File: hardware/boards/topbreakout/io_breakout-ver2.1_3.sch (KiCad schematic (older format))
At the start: 5 parts, among them J1 WURTH_ELECTRONICS_61400413321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, J2 MOLEX_52892-3033MOLEX_52892-3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, J3 USB-A-S-X-X-VT

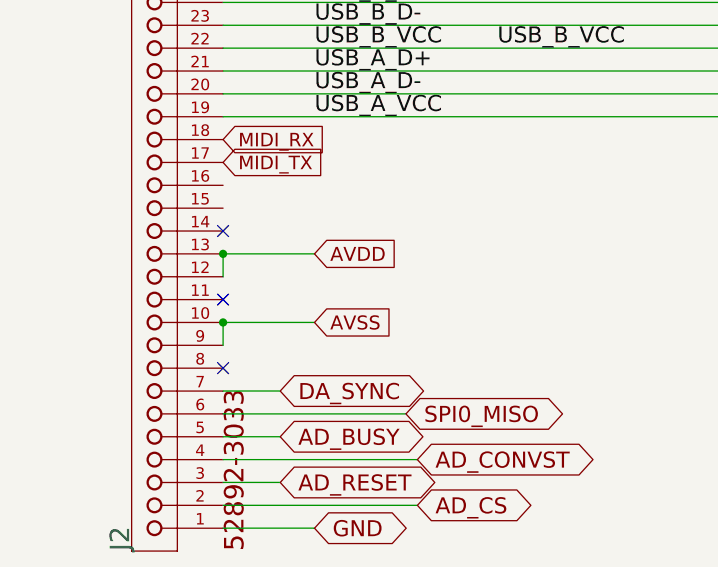
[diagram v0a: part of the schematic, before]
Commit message: refactor
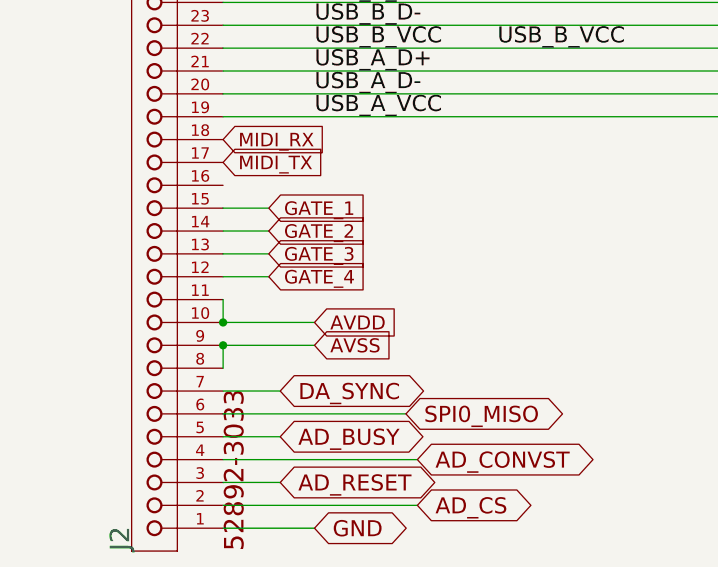
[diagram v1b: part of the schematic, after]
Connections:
- net AVDD: now also J2.10, J2.11; no longer J2.12, J2.13
- net AVSS: now also J2.8; no longer J2.10
- net GATE_2: now reaches J2.14
- net GATE_1: now reaches J2.15
- new net GATE_3: J2.13
- new net GATE_4: J2.12
- no-connect marks 3 -> 0
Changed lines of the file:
@@
-$EndComp
-$Comp
-L TopBreakout-eagle-import:MOLEX_52892-3033MOLEX_52892-3033_0_0 J2
-U 1 1 F1780596
-P 800 6100
-AR Path="/F1780596" Ref="J2"  Part="1"
-AR Path="/5D7F42FA/F1780596" Ref="J2"  Part="1"
-F 0 "J2" H 800 6000 85  0000 L TNN
-F 1 "MOLEX_52892-3033MOLEX_52892-3033_0_0" H 800 6100 50  0001 C CNN
-F 2 "topbreakout:MOLEX_52892-3033_0" H 800 6100 50  0001 C CNN
-F 3 "" H 800 6100 50  0001 C CNN
-	1    800  6100
-	0    -1   -1   0
 $EndComp
 $Comp
@@
 Wire Wire Line
 	5000 5800 6100 5800
-Wire Wire Line
-	1400 5200 1400 5100
-Wire Wire Line
-	1400 4900 1400 4800
-Wire Wire Line
-	1400 4800 1800 4800
-Connection ~ 1400 4800
-Wire Wire Line
-	1400 5100 1800 5100
-Connection ~ 1400 5100
-NoConn ~ 1400 5300
-NoConn ~ 1400 5000
-NoConn ~ 1400 4700
-Text GLabel 1800 4800 2    61   Input ~ 0
+Text GLabel 1800 5100 2    61   Input ~ 0
 AVDD
-Text GLabel 1800 5100 2    61   Input ~ 0
+Text GLabel 1800 5200 2    61   Input ~ 0
 AVSS
 Text GLabel 1400 4300 2    59   Input ~ 0
@@
 Text GLabel 1400 4400 2    59   Input ~ 0
 MIDI_TX
+$Comp
+L TopBreakout-eagle-import:MOLEX_52892-3033MOLEX_52892-3033_0_0 J2
+U 1 1 F1780596
+P 800 6100
+AR Path="/F1780596" Ref="J2"  Part="1"
+AR Path="/5D7F42FA/F1780596" Ref="J2"  Part="1"
+F 0 "J2" H 800 6000 85  0000 L TNN
+F 1 "MOLEX_52892-3033MOLEX_52892-3033_0_0" H 800 6100 50  0001 C CNN
+F 2 "topbreakout:MOLEX_52892-3033_0" H 800 6100 50  0001 C CNN
+F 3 "" H 800 6100 50  0001 C CNN
+	1    800  6100
+	0    -1   -1   0
+$EndComp
+Wire Wire Line
+	1400 5300 1400 5200
+Connection ~ 1400 5200
+Wire Wire Line
+	1400 5200 1800 5200
+Wire Wire Line
+	1800 5100 1400 5100
+Wire Wire Line
+	1400 5000 1400 5100
+Connection ~ 1400 5100
+Wire Wire Line
+	1400 4900 1600 4900
+Wire Wire Line
+	1400 4800 1600 4800
+Wire Wire Line
+	1400 4700 1600 4700
+Wire Wire Line
+	1400 4600 1600 4600
+Text GLabel 1600 4600 2    59   Input ~ 0
+GATE_1
+Text GLabel 1600 4700 2    59   Input ~ 0
+GATE_2
+Text GLabel 1600 4800 2    59   Input ~ 0
+GATE_3
+Text GLabel 1600 4900 2    59   Input ~ 0
+GATE_4
 $EndSCHEMATC

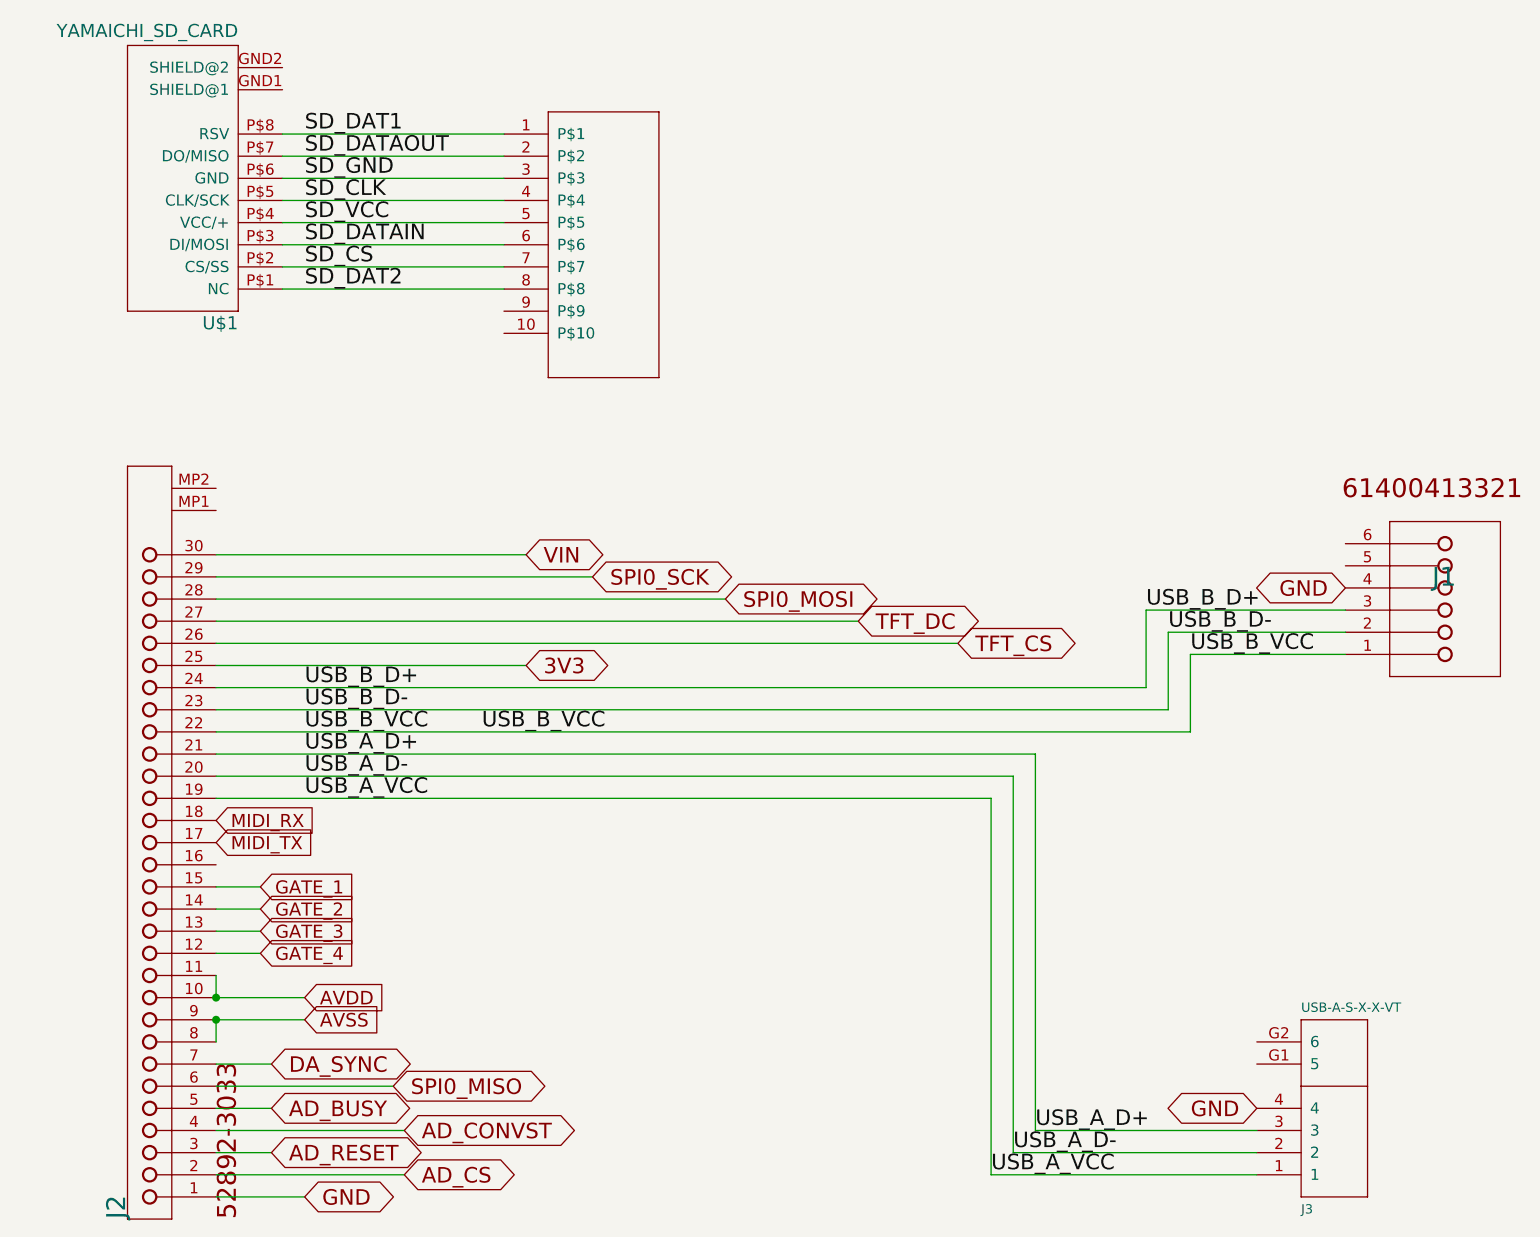
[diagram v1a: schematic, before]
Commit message: routed, ERC checks success
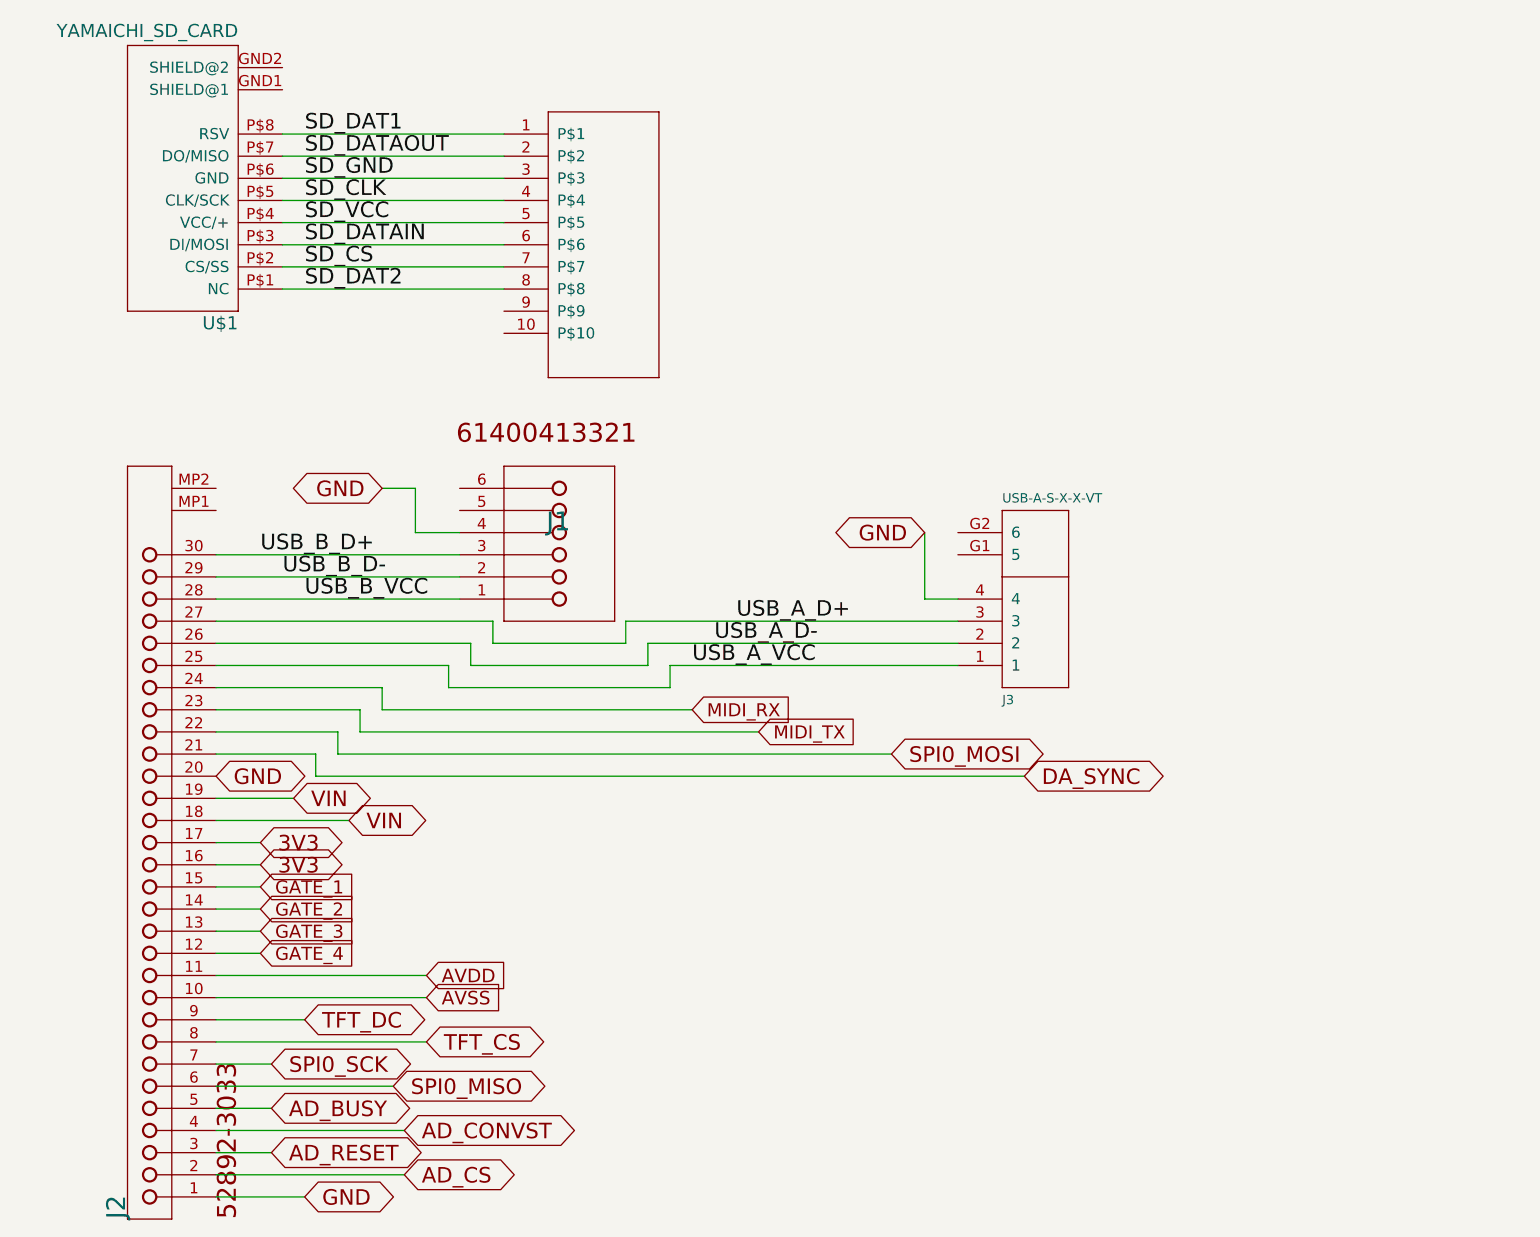
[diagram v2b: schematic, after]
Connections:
- net 3V3: now also J2.16, J2.17; no longer J2.25
- net AVDD: no longer J2.10
- net AVSS: now also J2.10; no longer J2.8, J2.9
- net DA_SYNC: now also J2.21; no longer J2.7
- net GND: now also J2.20
- net MIDI_RX: now also J2.24; no longer J2.18
- net MIDI_TX: now also J2.23; no longer J2.17
- net SPI0_MOSI: now also J2.22; no longer J2.28
- net SPI0_SCK: now also J2.7; no longer J2.29
- net TFT_CS: now also J2.8; no longer J2.26
- net TFT_DC: now also J2.9; no longer J2.27
- net USB_A_D+: now also J2.27; no longer J2.21
- net USB_A_D-: now also J2.26; no longer J2.20
- net USB_A_VCC: now also J2.25; no longer J2.19
- net USB_B_D+: now also J2.30; no longer J2.24
- net USB_B_D-: now also J2.29; no longer J2.23
- net USB_B_VCC: now also J2.28; no longer J2.22
- net VIN: now also J2.18, J2.19; no longer J2.30
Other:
- moved on the sheet: J1, J3
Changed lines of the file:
@@
 Comment4 ""
 $EndDescr
-Wire Wire Line
-	6500 3550 5800 3550
-Wire Wire Line
-	5800 3550 5800 3900
-Wire Wire Line
-	5800 3900 1400 3900
-Text Label 5800 3550 0    70   ~ 0
+Text Label 1800 3300 0    70   ~ 0
 USB_B_VCC
-Text Label 2600 3900 0    70   ~ 0
-USB_B_VCC
-Text Label 1800 3900 0    70   ~ 0
-USB_B_VCC
-Wire Wire Line
-	6500 3450 5700 3450
-Wire Wire Line
-	5700 3450 5700 3800
-Wire Wire Line
-	5700 3800 1400 3800
-Text Label 5700 3450 0    70   ~ 0
+Text Label 1700 3200 0    70   ~ 0
 USB_B_D-
-Text Label 1800 3800 0    70   ~ 0
-USB_B_D-
-Wire Wire Line
-	6500 3350 5600 3350
-Wire Wire Line
-	5600 3350 5600 3700
-Wire Wire Line
-	5600 3700 1400 3700
-Text Label 5600 3350 0    70   ~ 0
+Text Label 1600 3100 0    70   ~ 0
 USB_B_D+
-Text Label 1800 3700 0    70   ~ 0
-USB_B_D+
-Text GLabel 6100 5600 0    70   BiDi ~ 0
-GND
-Text GLabel 6500 3250 0    70   BiDi ~ 0
+Text GLabel 4600 3000 0    70   BiDi ~ 0
+GND
+Text GLabel 2150 2800 0    70   BiDi ~ 0
 GND
 Wire Wire Line
 	1400 6000 1800 6000
-Text GLabel 1800 6000 2    70   BiDi ~ 0
-GND
-Wire Wire Line
-	4900 5900 4900 4200
-Wire Wire Line
-	4900 4200 1400 4200
-Text Label 4900 5900 0    70   ~ 0
+Text GLabel 1400 4100 2    70   BiDi ~ 0
+GND
+Text Label 3550 3600 0    70   ~ 0
 USB_A_VCC
-Text Label 1800 4200 0    70   ~ 0
-USB_A_VCC
-Wire Wire Line
-	5100 5700 5100 4000
-Wire Wire Line
-	5100 4000 1400 4000
-Text Label 5100 5700 0    70   ~ 0
+Text Label 3750 3400 0    70   ~ 0
 USB_A_D+
-Text Label 1800 4000 0    70   ~ 0
-USB_A_D+
-Wire Wire Line
-	1400 3500 4750 3500
-Text GLabel 4750 3500 2    70   BiDi ~ 0
+Text GLabel 2350 5300 2    70   BiDi ~ 0
 TFT_CS
-Wire Wire Line
-	1400 3400 4300 3400
-Text GLabel 4300 3400 2    70   BiDi ~ 0
+Text GLabel 1800 5200 2    70   BiDi ~ 0
 TFT_DC
-Wire Wire Line
-	1400 3200 3100 3200
-Text GLabel 3100 3200 2    70   BiDi ~ 0
+Text GLabel 1650 5400 2    70   BiDi ~ 0
 SPI0_SCK
-Wire Wire Line
-	1400 3300 3700 3300
-Text GLabel 3700 3300 2    70   BiDi ~ 0
+Text GLabel 4450 4000 2    70   BiDi ~ 0
 SPI0_MOSI
 Wire Wire Line
-	1400 3100 2800 3100
-Text GLabel 2800 3100 2    70   BiDi ~ 0
+	2150 3800 3550 3800
+Text GLabel 1750 4200 2    70   BiDi ~ 0
 VIN
-Wire Wire Line
-	1400 4100 5000 4100
-Wire Wire Line
-	5000 4100 5000 5800
-Text Label 5000 5800 0    70   ~ 0
-USB_A_D-
-Text Label 1800 4100 0    70   ~ 0
+Text Label 3650 3500 0    70   ~ 0
 USB_A_D-
 Wire Wire Line
@@
 Wire Wire Line
 	1400 5400 1650 5400
-Text GLabel 1650 5400 2    70   BiDi ~ 0
+Text GLabel 5050 4100 2    70   BiDi ~ 0
 DA_SYNC
-Wire Wire Line
-	1400 3600 2800 3600
-Text GLabel 2800 3600 2    70   BiDi ~ 0
+Text GLabel 1600 4500 2    70   BiDi ~ 0
 3V3
 $Comp
 L TopBreakout-eagle-import:WURTH_ELECTRONICS_61400413321WURTH_ELECTRONICS_61400413321_0_0 J1
 U 1 1 92202B0B
-P 7100 3350
+P 3100 3100
 AR Path="/92202B0B" Ref="J1"  Part="1"
 AR Path="/5D7F42FA/92202B0B" Ref="J1"  Part="1"
-F 0 "J1" H 7200 3250 85  0000 L TNN
-F 1 "WURTH_ELECTRONICS_61400413321WURTH_ELECTRONICS_61400413321_0_0" H 7100 3350 50  0001 C CNN
-F 2 "topbreakout:WURTH_ELECTRONICS_61400413321_0" H 7100 3350 50  0001 C CNN
-F 3 "" H 7100 3350 50  0001 C CNN
-	1    7100 3350
+F 0 "J1" H 3200 3000 85  0000 L TNN
+F 1 "WURTH_ELECTRONICS_61400413321WURTH_ELECTRONICS_61400413321_0_0" H 3100 3100 50  0001 C CNN
+F 2 "topbreakout:WURTH_ELECTRONICS_61400413321_0" H 3100 3100 50  0001 C CNN
+F 3 "" H 3100 3100 50  0001 C CNN
+	1    3100 3100
 	-1   0    0    1
 $EndComp
@@
 L TopBreakout-eagle-import:USB-A-S-X-X-VT J3
 U 1 1 83A3164B
-P 6100 5900
+P 4750 3600
 AR Path="/83A3164B" Ref="J3"  Part="1"
 AR Path="/5D7F42FA/83A3164B" Ref="J3"  Part="1"
-F 0 "J3" H 6300 6031 42  0000 L BNN
-F 1 "USB-A-S-X-X-VT" H 6300 5120 42  0000 L BNN
-F 2 "topbreakout:USB-A-S-X-X-VT" H 6100 5900 50  0001 C CNN
-F 3 "" H 6100 5900 50  0001 C CNN
-	1    6100 5900
+F 0 "J3" H 4950 3731 42  0000 L BNN
+F 1 "USB-A-S-X-X-VT" H 4950 2820 42  0000 L BNN
+F 2 "topbreakout:USB-A-S-X-X-VT" H 4750 3600 50  0001 C CNN
+F 3 "" H 4750 3600 50  0001 C CNN
+	1    4750 3600
 	1    0    0    1
 $EndComp
@@
 	-1   0    0    -1
 $EndComp
-Wire Wire Line
-	6100 5900 4900 5900
-Wire Wire Line
-	5100 5700 6100 5700
-Wire Wire Line
-	5000 5800 6100 5800
-Text GLabel 1800 5100 2    61   Input ~ 0
+Text GLabel 2350 5000 2    61   Input ~ 0
 AVDD
-Text GLabel 1800 5200 2    61   Input ~ 0
+Text GLabel 2350 5100 2    61   Input ~ 0
 AVSS
-Text GLabel 1400 4300 2    59   Input ~ 0
+Text GLabel 3550 3800 2    59   Input ~ 0
 MIDI_RX
-Text GLabel 1400 4400 2    59   Input ~ 0
+Text GLabel 3850 3900 2    59   Input ~ 0
 MIDI_TX
 $Comp
@@
 $EndComp
 Wire Wire Line
-	1400 5300 1400 5200
-Connection ~ 1400 5200
-Wire Wire Line
 	1400 5200 1800 5200
-Wire Wire Line
-	1800 5100 1400 5100
-Wire Wire Line
-	1400 5000 1400 5100
-Connection ~ 1400 5100
 Wire Wire Line
 	1400 4900 1600 4900
@@
 Text GLabel 1600 4900 2    59   Input ~ 0
 GATE_4
+Wire Wire Line
+	2350 5300 1400 5300
+Wire Wire Line
+	4600 3000 4600 3300
+Wire Wire Line
+	4600 3300 4750 3300
+Wire Wire Line
+	2500 3000 2300 3000
+Wire Wire Line
+	2300 3000 2300 2800
+Wire Wire Line
+	2300 2800 2150 2800
+Wire Wire Line
+	1400 5000 2350 5000
+Wire Wire Line
+	1400 5100 2350 5100
+Text GLabel 1800 6000 2    70   BiDi ~ 0
+GND
+Wire Wire Line
+	1400 4500 1600 4500
+Wire Wire Line
+	1600 4400 1400 4400
+Wire Wire Line
+	1400 3300 2500 3300
+Wire Wire Line
+	1400 3200 2500 3200
+Wire Wire Line
+	1400 3100 2500 3100
+Wire Wire Line
+	3250 3400 3250 3500
+Wire Wire Line
+	3250 3500 2650 3500
+Wire Wire Line
+	2650 3500 2650 3400
+Wire Wire Line
+	2650 3400 1400 3400
+Wire Wire Line
+	3350 3500 3350 3600
+Wire Wire Line
+	3350 3600 2550 3600
+Wire Wire Line
+	2550 3600 2550 3500
+Wire Wire Line
+	2550 3500 1400 3500
+Wire Wire Line
+	3450 3600 3450 3700
+Wire Wire Line
+	3450 3700 2450 3700
+Wire Wire Line
+	2450 3700 2450 3600
+Wire Wire Line
+	2450 3600 1400 3600
+Wire Wire Line
+	3450 3600 4750 3600
+Wire Wire Line
+	3350 3500 4750 3500
+Wire Wire Line
+	3250 3400 4750 3400
+Wire Wire Line
+	2150 3800 2150 3700
+Wire Wire Line
+	2150 3700 1400 3700
+Wire Wire Line
+	2050 3900 2050 3800
+Wire Wire Line
+	2050 3800 1400 3800
+Wire Wire Line
+	2050 3900 3850 3900
+Wire Wire Line
+	1950 4000 1950 3900
+Wire Wire Line
+	1950 3900 1400 3900
+Wire Wire Line
+	1950 4000 4450 4000
+Wire Wire Line
+	1850 4100 1850 4000
+Wire Wire Line
+	1850 4000 1400 4000
+Wire Wire Line
+	1850 4100 5050 4100
+Wire Wire Line
+	1400 4200 1750 4200
+Wire Wire Line
+	1400 4300 2000 4300
+Text GLabel 2000 4300 2    70   BiDi ~ 0
+VIN
+Text GLabel 1600 4400 2    70   BiDi ~ 0
+3V3
 $EndSCHEMATC

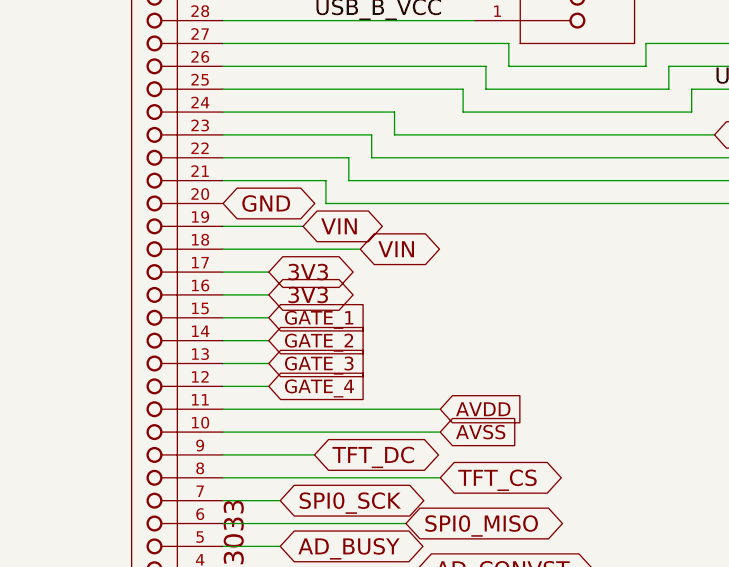
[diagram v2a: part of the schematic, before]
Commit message: revision 1.4 changes
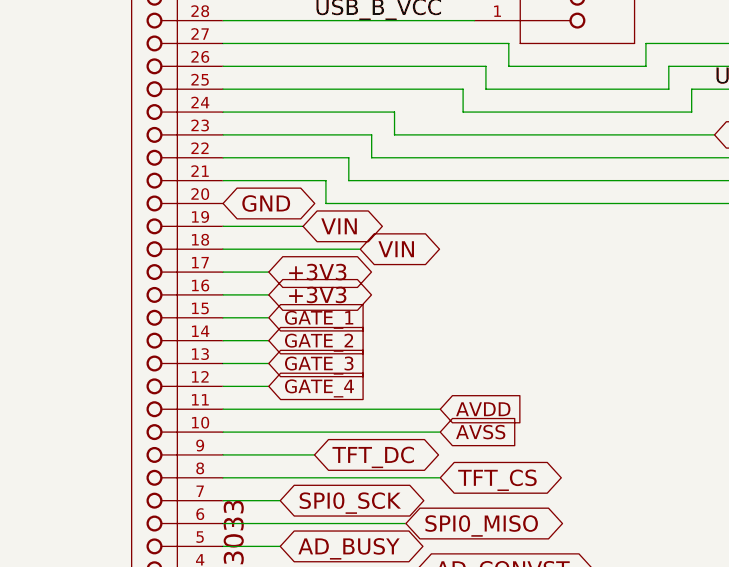
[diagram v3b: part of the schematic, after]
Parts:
- U$2: footprint topbreakout:TE_1-1734592-8 -> common:HFW8R-1STE1LF
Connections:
- net 3V3 renamed +3V3
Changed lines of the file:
@@
-EESchema Schematic File Version 4
-LIBS:TopBreakout-cache
+EESchema Schematic File Version 5
 EELAYER 30 0
 EELAYER END
@@
 Comment3 ""
 Comment4 ""
+Comment5 ""
+Comment6 ""
+Comment7 ""
+Comment8 ""
+Comment9 ""
 $EndDescr
 Text Label 1800 3300 0    70   ~ 0
@@
 DA_SYNC
 Text GLabel 1600 4500 2    70   BiDi ~ 0
-3V3
++3V3
 $Comp
 L TopBreakout-eagle-import:WURTH_ELECTRONICS_61400413321WURTH_ELECTRONICS_61400413321_0_0 J1
@@
 F 0 "U$2" H 2200 1800 50  0001 C CNN
 F 1 "1734592-8" H 2200 1800 50  0001 C CNN
-F 2 "topbreakout:TE_1-1734592-8" H 2200 1800 50  0001 C CNN
+F 2 "common:HFW8R-1STE1LF" H 2200 1800 50  0001 C CNN
 F 3 "" H 2200 1800 50  0001 C CNN
 	1    2200 1800
@@
 VIN
 Text GLabel 1600 4400 2    70   BiDi ~ 0
-3V3
++3V3
 $EndSCHEMATC
